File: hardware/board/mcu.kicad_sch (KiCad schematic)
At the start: 41 parts, among them J1 USB_B_Micro, J2 SM03B-SRSS-TB, J3 MidiIn, J4 MidiOut, SW101 SW_Push, SW102 SW_Push, U1 NCP1117-3.3_SOT223, U2 RP2350_80QFN, U4 THB001P, Y1 ABM8-272-T3

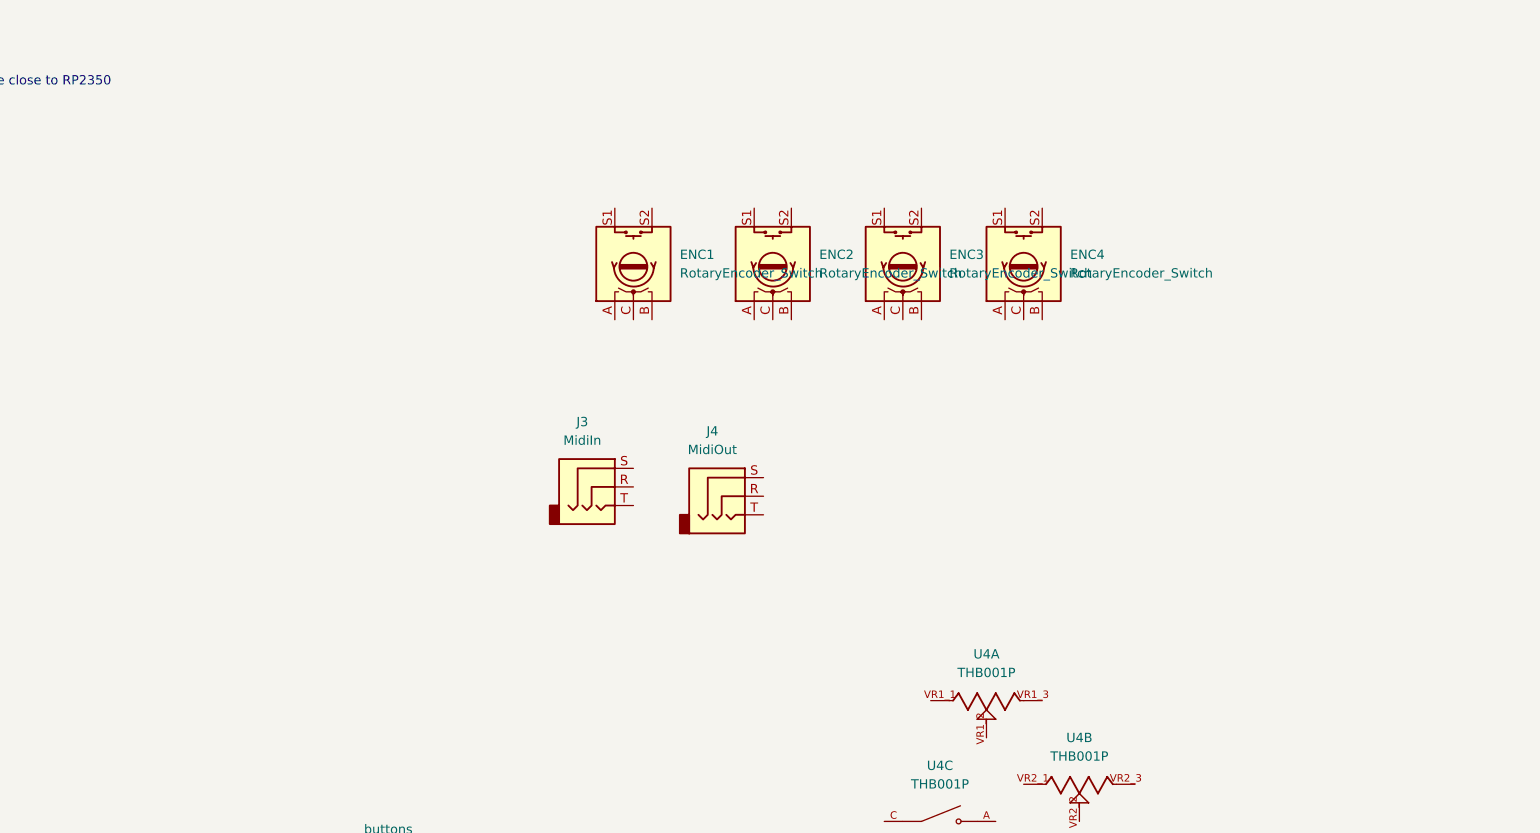
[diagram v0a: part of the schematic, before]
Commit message: encoder
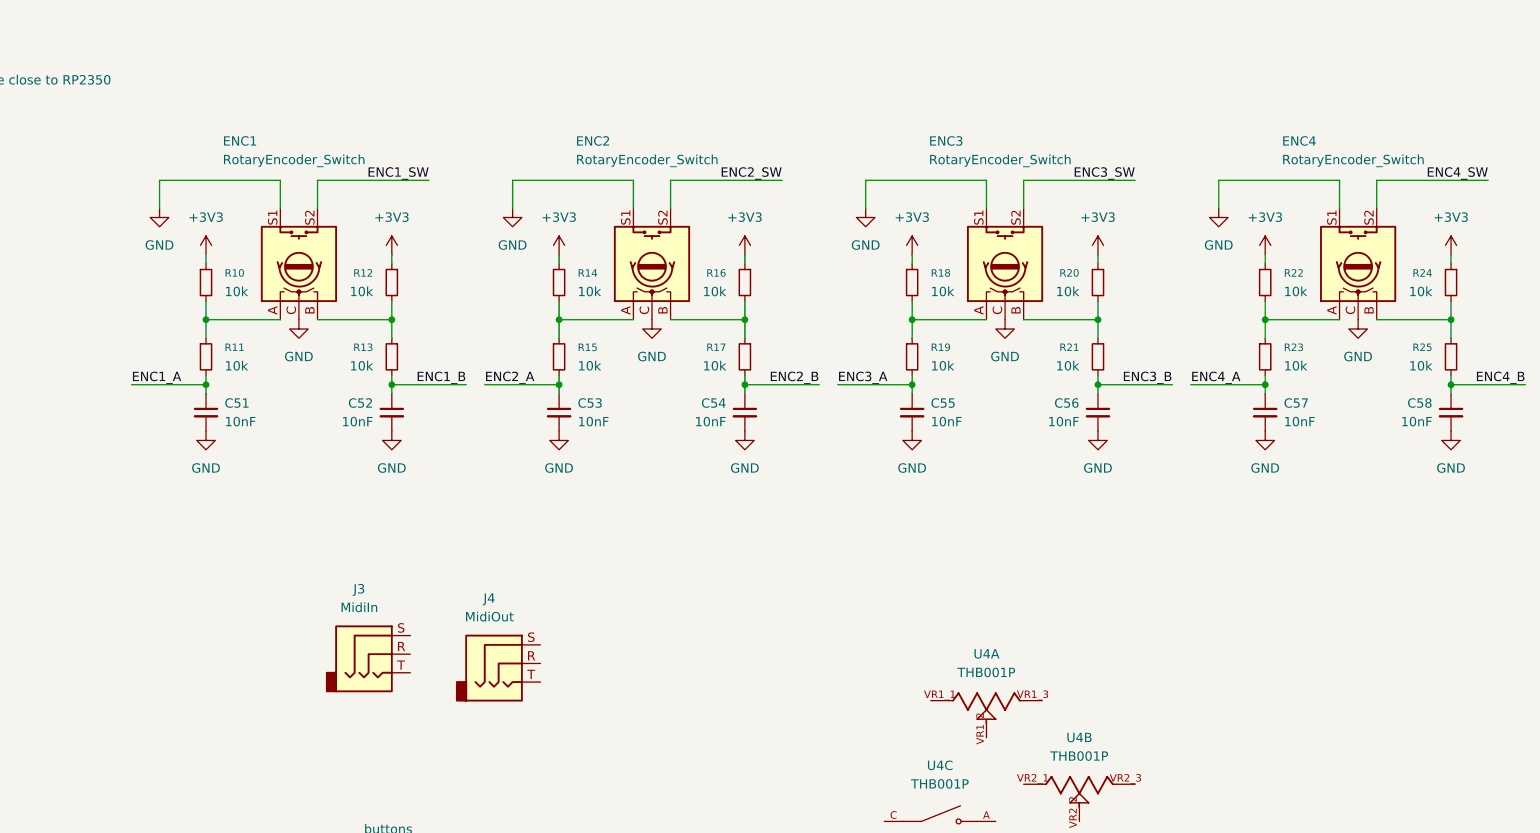
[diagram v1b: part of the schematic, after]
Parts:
- added C51, C52, C53, C54, C55, C56, C57, C58: 10nF, symbol Device:C_Small
- added R10, R11, R12, R13, R14, R15, R16, R17, R18, R19, R20, R21, R22, R23, R24, R25: 10k, symbol Device:R_Small
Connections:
- net +3V3: now also R10.1, R12.1, R14.1, R16.1, R18.1, R20.1, R22.1, R24.1
- net GND: now also ENC1.C, ENC1.S1, ENC2.C, ENC2.S1, ENC3.C, ENC3.S1, ENC4.C, ENC4.S1, C51.2, C52.2, C53.2, C54.2, C55.2, C56.2, C57.2, C58.2
- net at ENC4.A: now also R22.2, R23.1
- net at ENC4.B: now also R24.2, R25.1
- net ENC4_SW: now reaches ENC4.S2
- net at ENC2.A: now also R14.2, R15.1
- net at ENC2.B: now also R16.2, R17.1
- net ENC2_SW: now reaches ENC2.S2
- net at ENC1.A: now also R10.2, R11.1
- net at ENC1.B: now also R12.2, R13.1
- net ENC1_SW: now reaches ENC1.S2
- net at ENC3.A: now also R18.2, R19.1
- net at ENC3.B: now also R20.2, R21.1
- net ENC3_SW: now reaches ENC3.S2
- new net ENC1_A: C51.1, R11.2
- new net ENC1_B: C52.1, R13.2
- new net ENC2_A: C53.1, R15.2
- new net ENC2_B: C54.1, R17.2
- new net ENC3_A: C55.1, R19.2
- new net ENC3_B: C56.1, R21.2
- new net ENC4_A: C57.1, R23.2
- new net ENC4_B: C58.1, R25.2
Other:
- moved on the sheet: ENC1, J3, J4
